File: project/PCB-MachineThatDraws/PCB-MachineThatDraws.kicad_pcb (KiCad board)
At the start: 2 copper layers, 60 x 60 mm, 29 parts, among them J1 SD_Card_Device, J10 Conn_02x03_Counter_Clockwise, J2 Barrel_Jack_Switch, J3 Switch, J4 Switch, J5 Moteur, J6 Moteur, J7 Arret urgence, J8 Servo-Moteur, J9 Conn_02x03_Counter_Clockwise, U1 ESP32-S3-UNO, U2 R-78E5.0-1.0

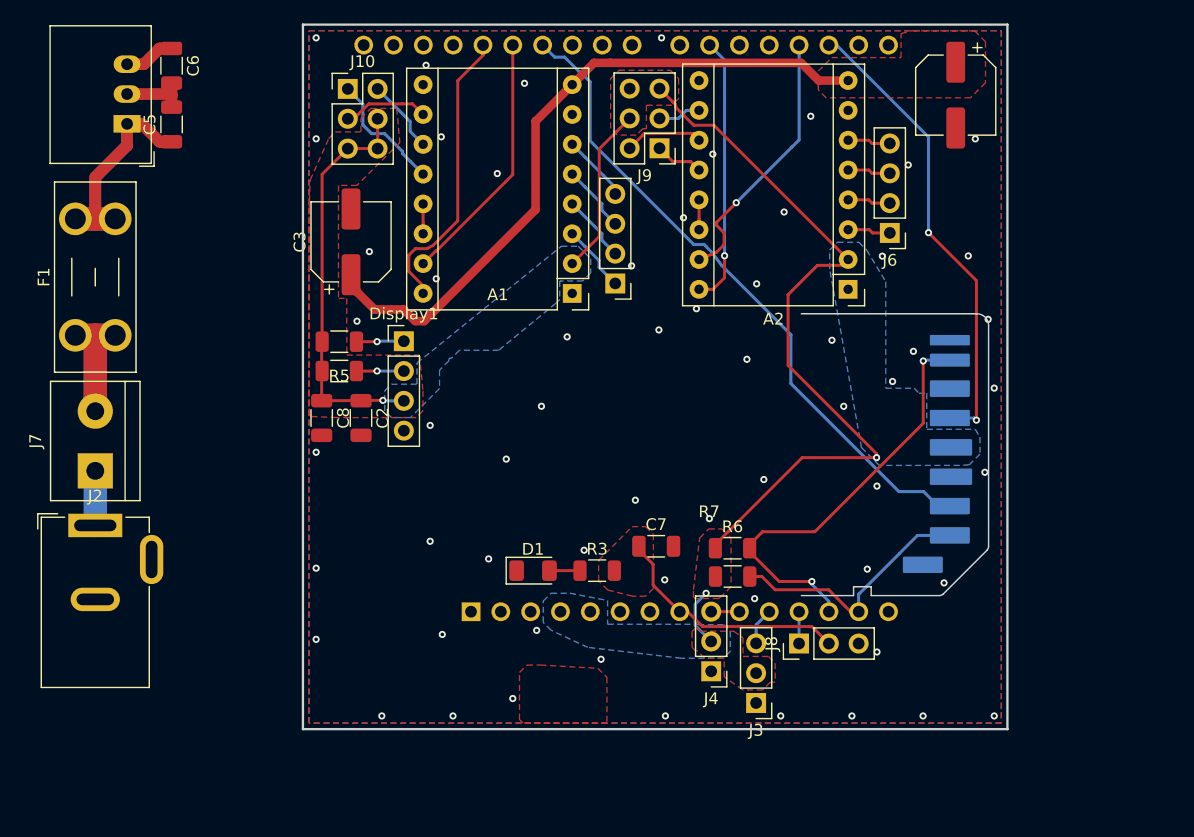
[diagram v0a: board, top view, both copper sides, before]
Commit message: Peut etre a revoir
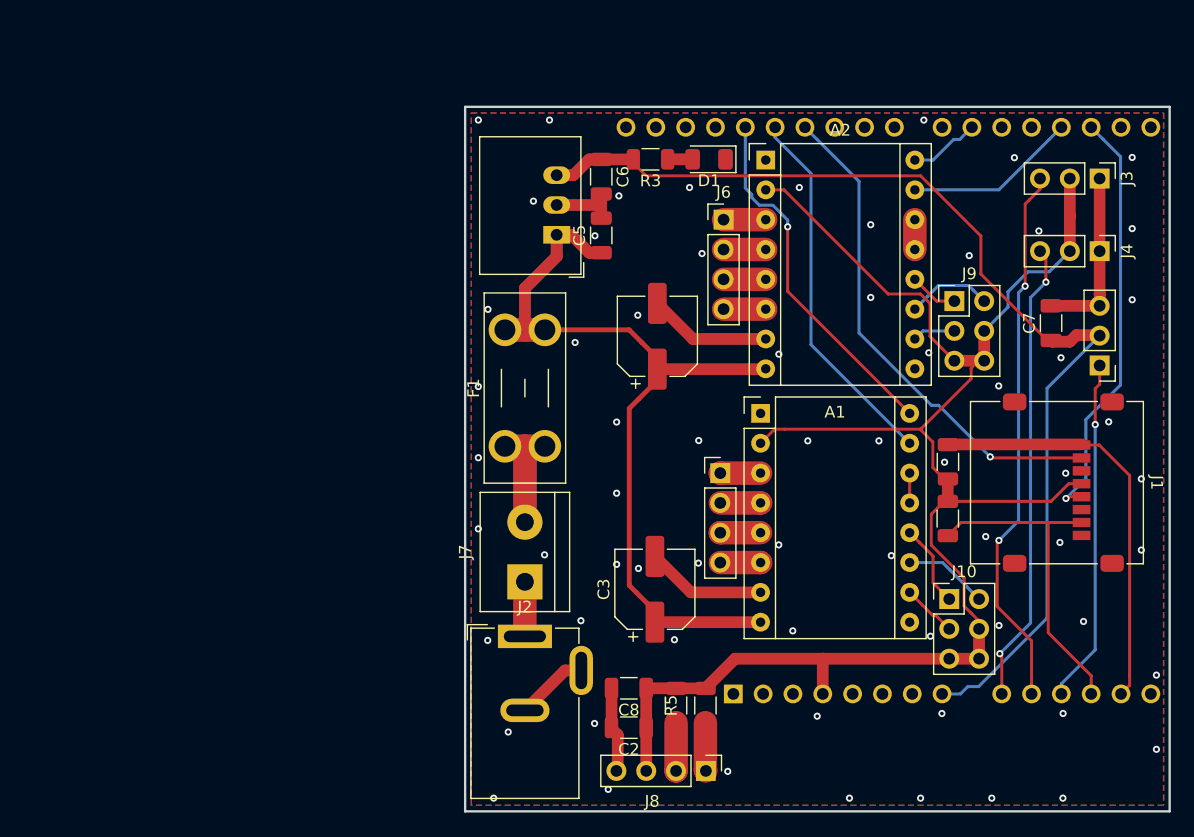
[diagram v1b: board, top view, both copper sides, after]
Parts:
- J1: footprint Connector_Card:SD_Card_Device_16mm_SlotDepth -> Connector_Card:microSD_HC_Molex_47219-2001
- moved J10 67.2 mm to (178.2, 111.9)
- moved J3 53.4 mm to (191.0, 76.1), turned to -90 degrees
- moved J4 48.7 mm to (191.0, 82.3), turned to -90 degrees
- moved Display1 44.7 mm to (157.5, 126.6), turned to -90 degrees
- moved R4 44.0 mm to (157.5, 121.0), turned to -90 degrees
- moved R5 40.4 mm to (155.0, 121.0), turned to -90 degrees
- moved C3 39.3 mm to (153.2, 111.1)
- moved C7 38.6 mm to (186.9, 88.4), turned to 90 degrees
- moved D1 38.1 mm to (157.8, 74.5), turned to 180 degrees
- moved U2 37.8 mm to (144.8, 80.9)
- moved C5 37.8 mm to (148.6, 81.0)
- moved C6 37.8 mm to (148.6, 76.0)
- moved J7 37.8 mm to (142.1, 110.5)
- moved F1 37.8 mm to (140.4, 98.9)
- moved J2 37.8 mm to (142.1, 115.1)
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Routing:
- net +5V: track 25.1 -> 93.0 mm
- net GND: track 5.88 -> 55.1 mm, vias 60 -> 66
- net D01: track 3.16 -> 46.6 mm, vias 0 -> 2
- net D02: track 2.41 -> 39.6 mm, vias 0 -> 2
- net D07: track 2.71 -> 29.3 mm, vias 0 -> 1
- net +3.3V: track 117.0 -> 142.5 mm, vias 3 -> 0
- net D03: track 22.9 -> 6.01 mm, vias 1 -> 0
- net D05: track 21.8 -> 35.5 mm
- net D11: track 56.3 -> 42.8 mm, vias 0 -> 1
- net D13: track 21.8 -> 31.7 mm
- net D19: track 36.7 -> 27.8 mm, vias 2 -> 0
- net D17: track 22.7 -> 14.7 mm, vias 1 -> 0
- net D12: track 24.9 -> 30.8 mm, vias 0 -> 1
- net +12V: track 88.2 -> 82.4 mm
- net D18: track 39.9 -> 36.0 mm, vias 2 -> 1
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- removed copper zone on F.Cu, net +12V
- removed copper zone on B.Cu, net +3.3V
- removed copper zone on F.Cu, net +3.3V
- removed copper zone on F.Cu, net +5V
